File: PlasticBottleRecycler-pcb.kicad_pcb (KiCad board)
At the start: 2 copper layers, 70.9 x 56.9 mm, 28 parts, among them J1 SWIM, J2 LCD, J3 Screw_Terminal_01x04, J4 NTC, J5 HEATER, J6 FAN1, J7 +12V, J8 +5V, Q1 IRF3205, Q2 BC337, SW1 RESET, SW2 SW_Push, SW3 SW_Push, SW4 SW_Push, U1 STM8S005K6T6C

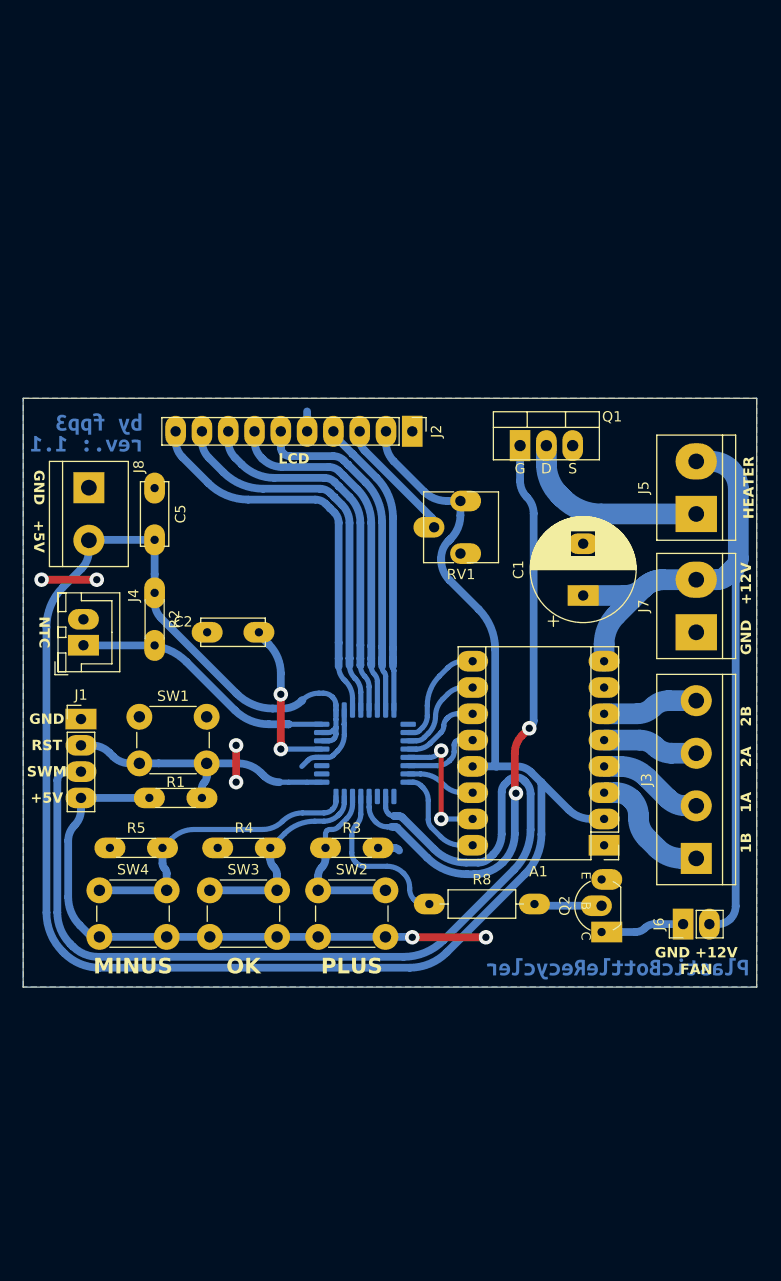
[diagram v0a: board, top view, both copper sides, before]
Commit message: Revision 2.0
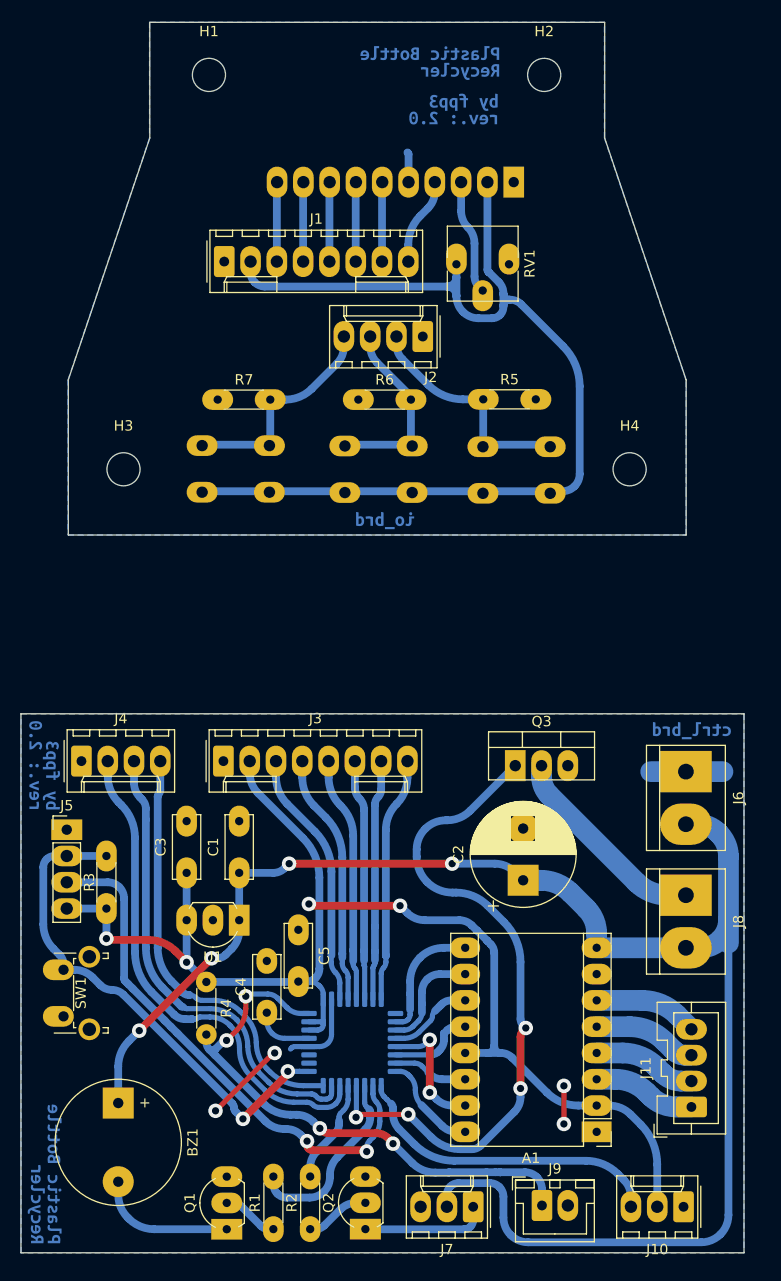
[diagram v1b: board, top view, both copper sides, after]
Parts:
- removed R8: 680, Resistor_THT:R_Axial_DIN0207_L6.3mm_D2.5mm_P10.16mm_Horizontal
- removed kibuzzard-679458C4: G***, kibuzzard-679458C4
- removed kibuzzard-67C1DC92: G***, kibuzzard-67C1DC92
- added BZ1: Buzzer, Buzzer_Beeper:Buzzer_12x9.5RM7.6, F.Cu at (124.3, 140.2)
- added C3: 100nF, Capacitor_THT:C_Disc_D6.0mm_W2.5mm_P5.00mm, F.Cu at (130.9, 118.0)
- added C4: 100n, Capacitor_THT:C_Disc_D6.0mm_W2.5mm_P5.00mm, F.Cu at (138.7, 131.5)
- added H1: MountingHole, MountingHole:MountingHole_3.2mm_M3, F.Cu at (133.1, 40.9)
- added H2: MountingHole, MountingHole:MountingHole_3.2mm_M3, F.Cu at (165.5, 40.9)
- added H3: MountingHole, MountingHole:MountingHole_3.2mm_M3, F.Cu at (124.8, 79.0)
- added H4: MountingHole, MountingHole:MountingHole_3.2mm_M3, F.Cu at (173.7, 79.0)
- added J10: RUNOUT, Connector_Molex:Molex_KK-254_AE-6410-03A_1x03_P2.54mm_Vertical, F.Cu at (178.9, 150.2)
- added J11: STEPPER, Connector_JST:JST_XA_B04B-XASK-1_1x04_P2.50mm_Vertical, F.Cu at (179.7, 140.6)
- added J12: LCD, Connector_PinHeader_2.54mm:PinHeader_1x10_P2.54mm_Vertical, B.Cu at (162.5, 51.3)
- added J9: NTC, Connector_JST:JST_XH_B2B-XH-A_1x02_P2.50mm_Vertical, F.Cu at (165.3, 150.1)
- added Q3: IRF3205, Package_TO_SOT_THT:TO-220-3_Vertical, F.Cu at (162.7, 107.6)
- added R6: 10K, Resistor_THT:R_Axial_DIN0204_L3.6mm_D1.6mm_P5.08mm_Horizontal, F.Cu at (147.5, 72.3)
- added R7: 10K, Resistor_THT:R_Axial_DIN0204_L3.6mm_D1.6mm_P5.08mm_Horizontal, F.Cu at (133.9, 72.3)
- added U2: STM8S005K6T6C, Package_QFP:LQFP-32_7x7mm_P0.8mm, B.Cu at (146.9, 134.4)
- added kibuzzard-67C39444: G***, kibuzzard-67C39444, B.Cu at (117.2, 107.6)
- added kibuzzard-67C39444: G***, kibuzzard-67C39444, B.Cu at (156.7, 44.2)
- added kibuzzard-67C39452: G***, kibuzzard-67C39452, B.Cu at (117.2, 147.1)
- added kibuzzard-67C39452: G***, kibuzzard-67C39452, B.Cu at (154.4, 39.8)
- added kibuzzard-67C3947F: G***, kibuzzard-67C3947F, B.Cu at (179.8, 104.2)
- added kibuzzard-67C3B0C4: G***, kibuzzard-67C3B0C4, B.Cu at (150.1, 83.9)
- C1: value 1000u -> 330nF; footprint Capacitor_THT:CP_Radial_D10.0mm_P5.00mm -> Capacitor_THT:C_Disc_D6.0mm_W2.5mm_P5.00mm
- C2: value 100n -> 1000u; footprint Capacitor_THT:C_Disc_D6.0mm_W2.5mm_P5.00mm -> Capacitor_THT:CP_Radial_D10.0mm_P5.00mm
- J1: value SWIM -> Conn_01x08; footprint Connector_PinHeader_2.54mm:PinHeader_1x04_P2.54mm_Vertical -> Connector_Molex:Molex_KK-254_AE-6410-08A_1x08_P2.54mm_Vertical
- J2: value LCD -> Conn_01x04; footprint Connector_PinHeader_2.54mm:PinHeader_1x10_P2.54mm_Vertical -> Connector_Molex:Molex_KK-254_AE-6410-04A_1x04_P2.54mm_Vertical
- J3: value Screw_Terminal_01x04 -> Conn_01x08; footprint TerminalBlock:TerminalBlock_bornier-4_P5.08mm -> Connector_Molex:Molex_KK-254_AE-6410-08A_1x08_P2.54mm_Vertical
- J4: value NTC -> Conn_01x04; footprint Connector_JST:JST_XH_B2B-XH-A_1x02_P2.50mm_Vertical -> Connector_Molex:Molex_KK-254_AE-6410-04A_1x04_P2.54mm_Vertical
- J5: value HEATER -> SWIM; footprint TerminalBlock:TerminalBlock_bornier-2_P5.08mm -> Connector_PinHeader_2.54mm:PinHeader_1x04_P2.54mm_Vertical
- J6: value FAN1 -> +12V; footprint Connector_PinHeader_2.54mm:PinHeader_1x02_P2.54mm_Vertical -> TerminalBlock:TerminalBlock_bornier-2_P5.08mm
- J7: value +12V -> FAN1; footprint TerminalBlock:TerminalBlock_bornier-2_P5.08mm -> Connector_Molex:Molex_KK-254_AE-6410-03A_1x03_P2.54mm_Vertical
- J8: value +5V -> HEATER
- Q1: value IRF3205 -> BC337; footprint PCM_Package_TO_SOT_THT_AKL:TO-220-3_Vertical_GDS -> Package_TO_SOT_THT:TO-92L_Inline_Wide
- Q2: footprint PCM_Package_TO_SOT_THT_AKL:TO-92_Inline_Wide_CBE -> Package_TO_SOT_THT:TO-92L_Inline_Wide
- R1: value 10K -> 680
- R2: value 4K7 -> 680
- R4: value 10K -> 4K7
- SW1: footprint Button_Switch_THT:SW_PUSH_6mm_H5mm -> Button_Switch_THT:SW_Tactile_SPST_Angled_PTS645Vx39-2LFS
- SW2: value SW_Push -> BTN_PLUS; footprint Button_Switch_THT:SW_PUSH_6mm_H5mm -> Button_Switch_THT:SW_PUSH_6mm_H7.3mm; moved to B.Cu
- SW3: value SW_Push -> BTN_OK; footprint Button_Switch_THT:SW_PUSH_6mm_H5mm -> Button_Switch_THT:SW_PUSH_6mm_H7.3mm; moved to B.Cu
- SW4: value SW_Push -> BTN_MINUS; footprint Button_Switch_THT:SW_PUSH_6mm_H5mm -> Button_Switch_THT:SW_PUSH_6mm_H7.3mm; moved to B.Cu
- U1: value STM8S005K6T6C -> LM7805_TO220; footprint Package_QFP:LQFP-32_7x7mm_P0.8mm -> Package_TO_SOT_THT:TO-92L_Inline_Wide; moved to F.Cu
- moved Q1 80.8 mm to (134.8, 152.4), turned to 90 degrees
- moved J8 69.8 mm to (179.2, 120.1)
- moved J5 68.0 mm to (119.4, 113.8), turned to 0 degrees
- moved J7 59.5 mm to (158.6, 150.2), turned to 180 degrees
- moved R2 58.4 mm to (142.9, 147.3)
- moved R5 56.4 mm to (159.6, 72.2)
- moved SW2 48.4 mm to (166.1, 76.8), turned to 180 degrees
- moved SW3 47.2 mm to (152.7, 76.7), turned to 180 degrees
- moved J3 46.6 mm to (134.5, 107.2), turned to 0 degrees
- moved J1 46.3 mm to (134.6, 58.9)
- moved SW4 46.0 mm to (138.9, 76.7), turned to 180 degrees
- moved C5 44.9 mm to (141.7, 123.5)
- moved C1 42.7 mm to (136.0, 118.0)
- moved R1 38.5 mm to (139.3, 147.3), turned to -90 degrees
- moved Q2 36.7 mm to (148.2, 152.4)
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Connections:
- A1 pad 1: GND -> /Controller Board/GND
- A1 pad 10: A4988_MS1 -> /Controller Board/A4988_MS1
- A1 pad 11: A4988_MS2 -> /Controller Board/A4988_MS2
- A1 pad 12: A4988_MS3 -> /Controller Board/A4988_MS3
- A1 pad 13: +5V -> /Controller Board/+5V
- A1 pad 14: A4988_SLP -> /Controller Board/A4988_SLP
- A1 pad 15: A4988_STP -> /Controller Board/A4988_STP
- A1 pad 16: A4988_DIR -> /Controller Board/A4988_DIR
- A1 pad 2: +5V -> /Controller Board/+5V
- A1 pad 7: GND -> /Controller Board/GND
- A1 pad 8: +12V -> /Controller Board/+12V
- A1 pad 9: A4988_ENA -> /Controller Board/A4988_ENA
- C1 pad 1: +12V -> /Controller Board/+12V
- C1 pad 2: GND -> /Controller Board/GND
- C2 pad 1: Net-(U1-VCAP) -> /Controller Board/+12V
- C2 pad 2: GND -> /Controller Board/GND
- C5 pad 1: GND -> /Controller Board/GND
- C5 pad 2: +5V -> /Controller Board/+5V
- J1 pad 1: GND -> /IO Board/GND
- J1 pad 2: RESET -> /IO Board/+5V
- J1 pad 3: SWIM -> /IO Board/LCD_D7
- J1 pad 4: +5V -> /IO Board/LCD_D6
- J2 pad 1: GND -> /IO Board/GND
- J2 pad 2: +5V -> /IO Board/BTN_PLUS
- J2 pad 3: Net-(J2-Pin_3) -> /IO Board/BTN_OK
- J2 pad 4: LCD_RS -> /IO Board/BTN_MINUS
- J3 pad 1: Net-(A1-1B) -> /Controller Board/GND
- J3 pad 2: Net-(A1-1A) -> /Controller Board/+5V
- J3 pad 3: Net-(A1-2A) -> /Controller Board/LCD_D7
- J3 pad 4: Net-(A1-2B) -> /Controller Board/LCD_D6
- J4 pad 1: Net-(J4-Pin_1) -> /Controller Board/GND
- J4 pad 2: GND -> /Controller Board/BTN_PLUS
- J5 pad 1: Net-(J5-Pin_1) -> /Controller Board/GND
- J5 pad 2: +12V -> /Controller Board/RESET
- J6 pad 1: Net-(J6-Pin_1) -> /Controller Board/GND
- J6 pad 2: +12V -> /Controller Board/+12V
- J7 pad 1: GND -> Net-(J7-Pin_1)
- J7 pad 2: +12V -> /Controller Board/+12V
- J8 pad 1: GND -> Net-(J8-Pin_1)
- J8 pad 2: +5V -> /Controller Board/+12V
- Q1 pad 1: HEATER -> Net-(BZ1--)
- Q1 pad 2: Net-(J5-Pin_1) -> Net-(Q1-B)
- Q1 pad 3: GND -> /Controller Board/GND
- Q2 pad 1: Net-(J6-Pin_1) -> Net-(J7-Pin_1)
- Q2 pad 3: GND -> /Controller Board/GND
- R1 pad 1: +5V -> /Controller Board/BUZZER
- R1 pad 2: RESET -> Net-(Q1-B)
- R2 pad 1: +5V -> /Controller Board/FAN1
- R2 pad 2: Net-(J4-Pin_1) -> Net-(Q2-B)
- R3 pad 1: BTN_PLUS -> /Controller Board/+5V
- R3 pad 2: GND -> /Controller Board/RESET
- R4 pad 1: GND -> /Controller Board/+5V
- R4 pad 2: BTN_OK -> Net-(J9-Pin_1)
- R5 pad 1: GND -> /IO Board/BTN_PLUS
- R5 pad 2: BTN_MINUS -> /IO Board/GND
- RV1 pad 1: +5V -> /IO Board/+5V
- RV1 pad 2: Net-(J2-Pin_3) -> Net-(J12-Pin_3)
- RV1 pad 3: GND -> /IO Board/GND
- SW1 pad 1: GND -> /Controller Board/GND
- SW1 pad 2: RESET -> /Controller Board/RESET
- SW2 pad 1: BTN_PLUS -> /IO Board/BTN_PLUS
- SW2 pad 2: +5V -> /IO Board/+5V
- SW3 pad 1: BTN_OK -> /IO Board/BTN_OK
- SW3 pad 2: +5V -> /IO Board/+5V
- SW4 pad 1: BTN_MINUS -> /IO Board/BTN_MINUS
- SW4 pad 2: +5V -> /IO Board/+5V
- U1 pad 1: RESET -> /Controller Board/+12V
- U1 pad 2: unconnected-(U1-PA1/OSCIN-Pad2) -> /Controller Board/GND
- U1 pad 3: unconnected-(U1-PA2/OSCOUT-Pad3) -> /Controller Board/+5V
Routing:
- net +5V: track 256.0 -> 0.00 mm, vias 2 -> 0
- net /Controller Board/+12V: track 0.00 -> 157.0 mm, vias 0 -> 4
- net /Controller Board/+5V: track 0.00 -> 129.1 mm, vias 0 -> 4
- net /IO Board/+5V: track 0.00 -> 104.3 mm
- net SWIM: track 97.5 -> 0.00 mm
- net +12V: track 76.0 -> 0.00 mm
- net /Controller Board/HEATER: track 0.00 -> 65.8 mm, vias 0 -> 4
- net HEATER: track 58.5 -> 0.00 mm, vias 2 -> 0
- net Net-(J9-Pin_1): track 0.00 -> 55.8 mm, vias 0 -> 4
- net /Controller Board/SWIM: track 0.00 -> 51.9 mm, vias 0 -> 2
- net /Controller Board/BTN_PLUS: track 0.00 -> 48.8 mm
- net /Controller Board/RESET: track 0.00 -> 48.3 mm, vias 0 -> 2
- net /Controller Board/BTN_OK: track 0.00 -> 45.4 mm
- net /Controller Board/BTN_MINUS: track 0.00 -> 41.4 mm
- net LCD_D7: track 38.8 -> 0.00 mm
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- added copper zone on B.Cu, net /Controller Board/GND
- added copper zone on B.Cu, net /IO Board/GND
- removed copper zone on B.Cu, net GND
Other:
- board size 70.9 x 56.9 mm -> 69.8 x 118.9 mm
- board text removed: "+5V"
- board text removed: "1B 1A 2A 2B"
- board text removed: "GND"
- board text removed: "GND +12V"
- board text removed: "GND +12V FAN"
- board text removed: "GND +5V"
- board text removed: "HEATER"
- board text removed: "MINUS"
- board text removed: "NTC"
- board text removed: "OK"
- board text removed: "PLUS"
- board text removed: "RST"
- board text removed: "SWM"
